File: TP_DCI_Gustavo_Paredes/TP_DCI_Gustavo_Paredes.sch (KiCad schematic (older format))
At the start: 12 parts, among them X701DB9F/90 DB9_Female, X702DB9M/90 DB9_Male

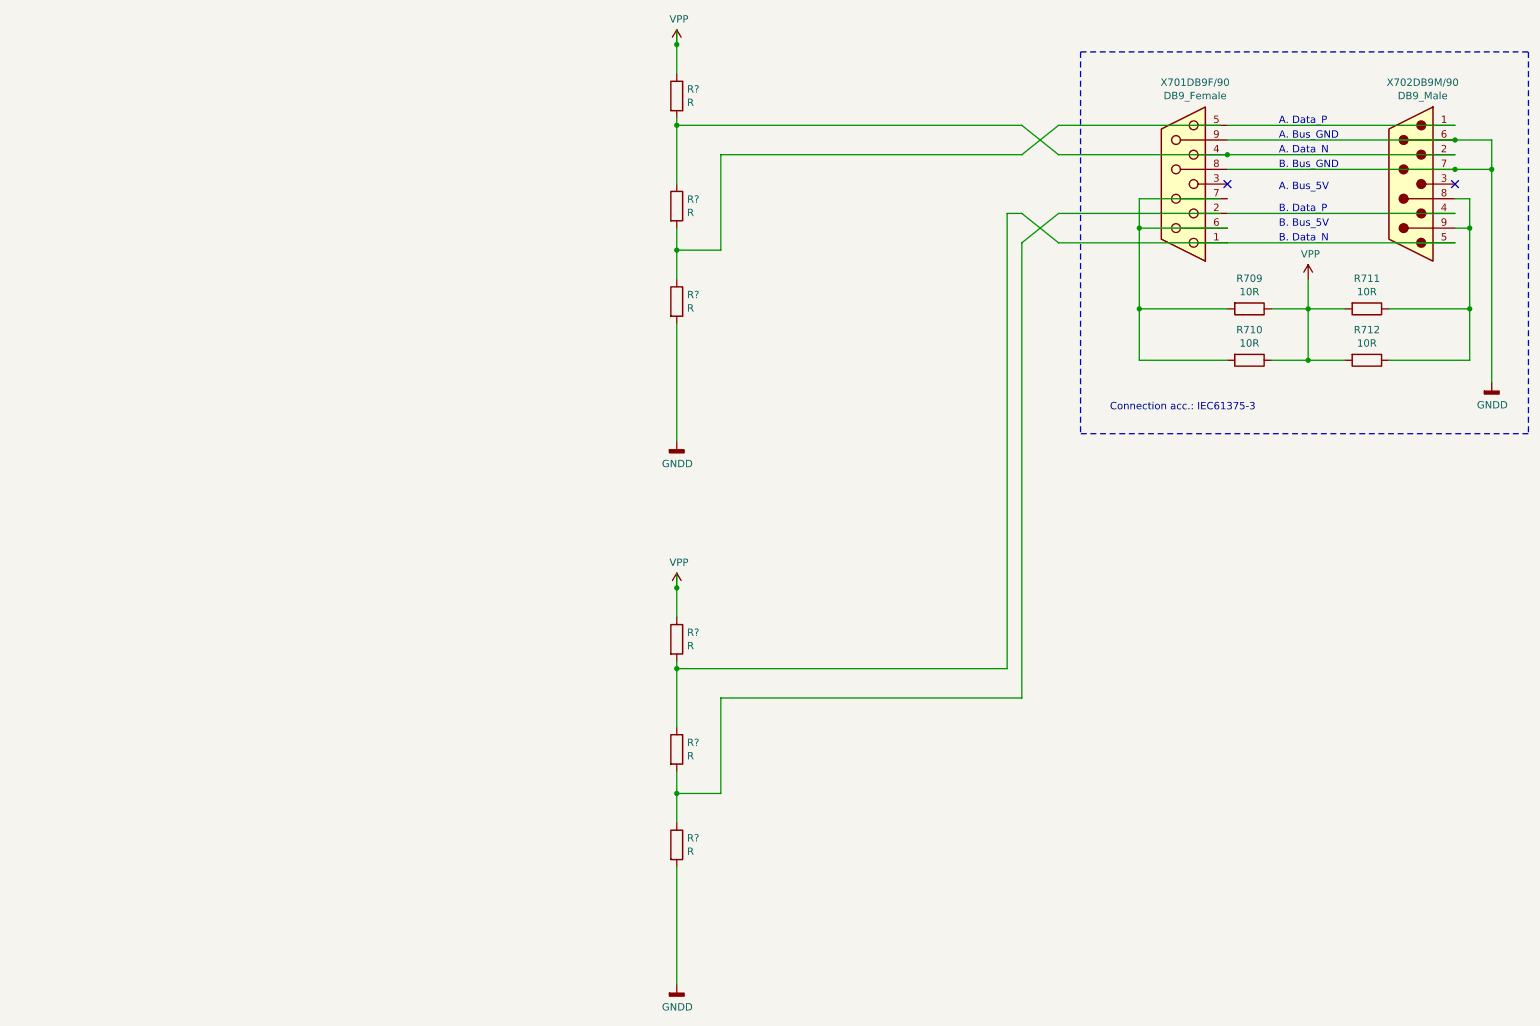
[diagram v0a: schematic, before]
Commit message: Saco Ejercicios Practica Clases
Saco a un carpeta externa los ejercicios de las clases.
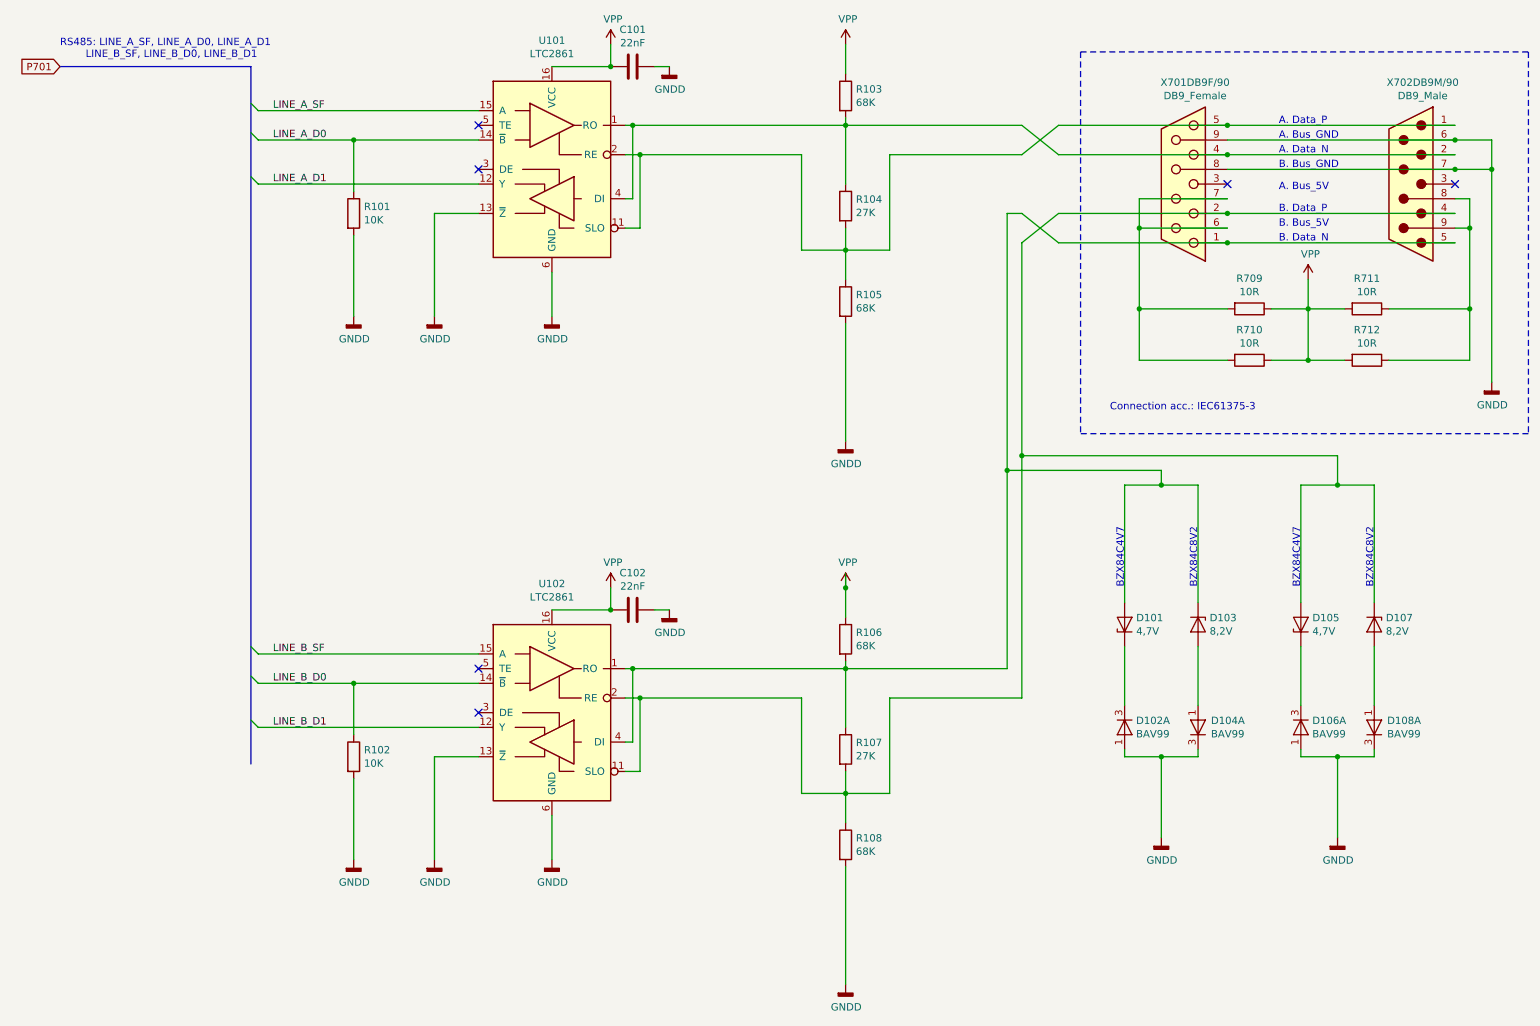
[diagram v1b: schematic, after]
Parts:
- added C101, C102: 22nF, symbol Device:C
- added D101, D105: 4,7V, symbol Device:D_Zener
- added D102, D104, D106, D108: BAV99, symbol Diode:BAV99
- added D103, D107: 8,2V, symbol Device:D_Zener
- added R101, R102: 10K, symbol Device:R
- added U101, U102: LTC2861, Package_SO:SSOP-28_5.3x10.2mm_P0.65mm, symbol Interface_UART:LTC2861
- R103, R105, R106, R108: renamed from R?; value R -> 68K
- R104, R107: renamed from R?; value R -> 27K
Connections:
- net labels added: LINE_A_D0, LINE_A_D1, LINE_A_SF, LINE_B_D0, LINE_B_D1, LINE_B_SF, P701
- wire segments 63 -> 140
- no-connect marks 2 -> 6
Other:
- note added: "BZX84C4V7"
- note added: "BZX84C8V2"
- note added: "RS485: LINE_A_SF, LINE_A_D0, LINE_A_D1\n LINE_B_SF, LINE_B_D0, LINE_B_D1"
- moved on the sheet: R103, R104, R105, R106, R107, R108
